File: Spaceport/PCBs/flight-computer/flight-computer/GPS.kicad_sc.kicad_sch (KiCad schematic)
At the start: 3 parts, among them U5 SAM-M10Q-00B

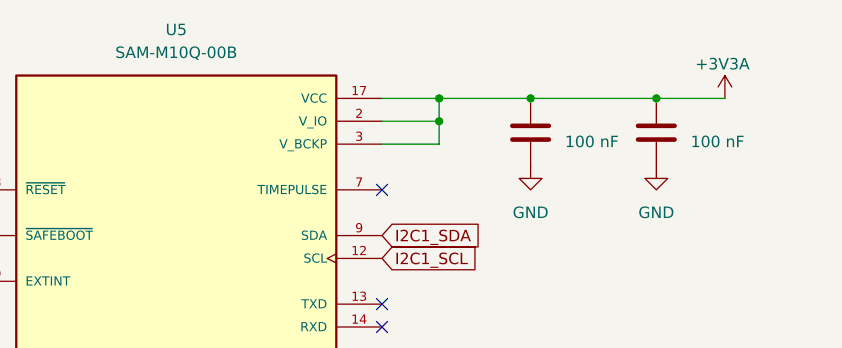
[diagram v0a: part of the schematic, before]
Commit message: Revert "Merge branch 'main' of https://github.com/Terrapin-Rocket-Team/SRAD-Avionics"
This reverts commit e5f68e4e525f2a5ad7eebbc917cc2807b67ca5e1, reversing
changes made to 8a40e2e341d8980ca528983581171a8bd9cc0146.
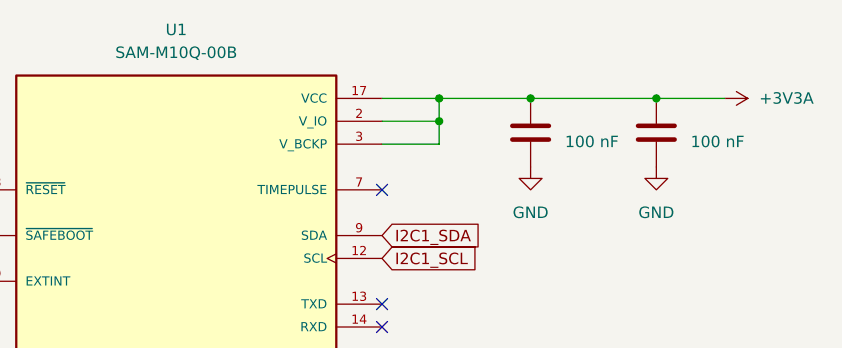
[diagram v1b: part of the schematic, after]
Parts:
- C18: footprint Capacitor_SMD:C_0603_1608Metric_Pad1.08x0.95mm_HandSolder -> (none)
- C?: renamed from C24; footprint Capacitor_SMD:C_0603_1608Metric_Pad1.08x0.95mm_HandSolder -> (none)
- U1: renamed from U5; footprint SAM-M10Q:XCVR_SAM-M10Q-00B -> SAM-M10Q-00B:XCVR_SAM-M10Q-00B
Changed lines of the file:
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@@
 		(on_board yes)
 		(dnp no)
-		(property "Reference" "C24"
+		(property "Reference" "C?"
 			(at 172.72 67.3099 0)
 			(effects
@@
 			)
 		)
-		(property "Footprint" "Capacitor_SMD:C_0603_1608Metric_Pad1.08x0.95mm_HandSolder"
+		(property "Footprint" ""
 			(at 169.8752 72.39 0)
 			(effects
@@
 			(project "flight-computer"
 				(path "/b419aaf0-5349-42bc-a414-d94cafbe45e9/d5f88fd8-f77f-45f2-a5f4-fb1e7853b7c3"
-					(reference "C24")
+					(reference "C?")
 					(unit 1)
 				)
@@
 			)
 		)
-		(property "Footprint" "Capacitor_SMD:C_0603_1608Metric_Pad1.08x0.95mm_HandSolder"
+		(property "Footprint" ""
 			(at 155.9052 72.39 0)
 			(effects
@@
 	(symbol
 		(lib_id "power:+3V3")
-		(at 176.53 64.77 0)
+		(at 176.53 64.77 270)
 		(unit 1)
 		(exclude_from_sim no)
@@
 		(on_board yes)
 		(dnp no)
+		(fields_autoplaced yes)
 		(property "Reference" "#PWR049"
-			(at 176.53 68.58 0)
+			(at 172.72 64.77 0)
 			(effects
 				(font
@@
 		)
 		(property "Value" "+3V3A"
-			(at 173.228 60.9599 0)
+			(at 180.34 64.7699 90)
 			(effects
 				(font
@@
 		(dnp no)
 		(fields_autoplaced yes)
-		(property "Reference" "U5"
+		(property "Reference" "U?"
 			(at 115.57 57.15 0)
 			(effects
@@
 			)
 		)
-		(property "Footprint" "SAM-M10Q:XCVR_SAM-M10Q-00B"
+		(property "Footprint" "SAM-M10Q-00B:XCVR_SAM-M10Q-00B"
 			(at 115.57 80.01 0)
 			(effects
@@
 			(project "flight-computer"
 				(path "/b419aaf0-5349-42bc-a414-d94cafbe45e9/d5f88fd8-f77f-45f2-a5f4-fb1e7853b7c3"
-					(reference "U5")
-					(unit 1)
-				)
+					(reference "U?")
+					(unit 1)
+				)
